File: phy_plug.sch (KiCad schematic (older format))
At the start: 20 parts, among them J6 HY951180A_RJ45, U1 KSZ8081

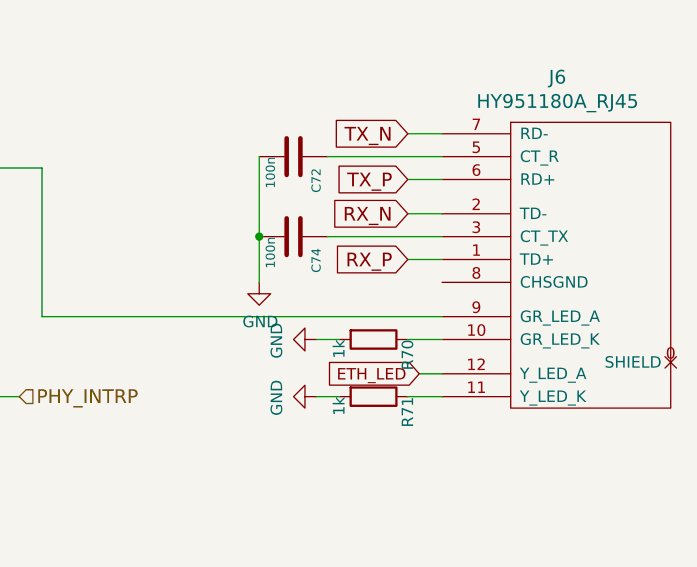
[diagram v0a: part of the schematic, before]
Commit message: small production changes
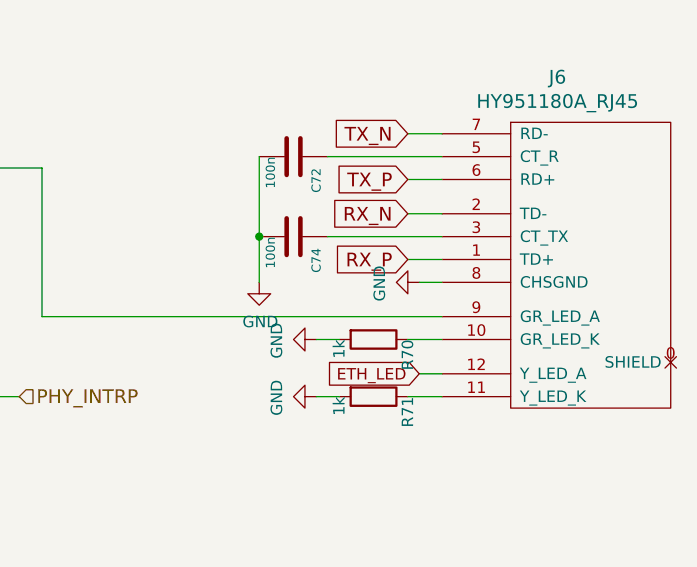
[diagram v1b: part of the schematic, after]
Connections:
- net GND: now also J6.8 (CHSGND)
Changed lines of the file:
@@
 Text GLabel 7350 4700 0    50   Input ~ 0
 ETH_LED
+$Comp
+L power:GND #PWR0199
+U 1 1 5D2D4E66
+P 7350 4300
+F 0 "#PWR0199" H 7350 4050 50  0001 C CNN
+F 1 "GND" H 7355 4127 50  0000 C CNN
+F 2 "" H 7350 4300 50  0000 C CNN
+F 3 "" H 7350 4300 50  0000 C CNN
+	1    7350 4300
+	0    1    1    0
+$EndComp
+Wire Wire Line
+	7350 4300 7450 4300
 $EndSCHEMATC
